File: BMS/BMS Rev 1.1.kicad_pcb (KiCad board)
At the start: 2 copper layers, 18 x 50.8 mm, 38 parts, among them J2 out, J3 out, J4 in, J5 in, Q1 CSD18502Q5B, Q2 CSD18502Q5B, U1 BQ41Z50RSNR

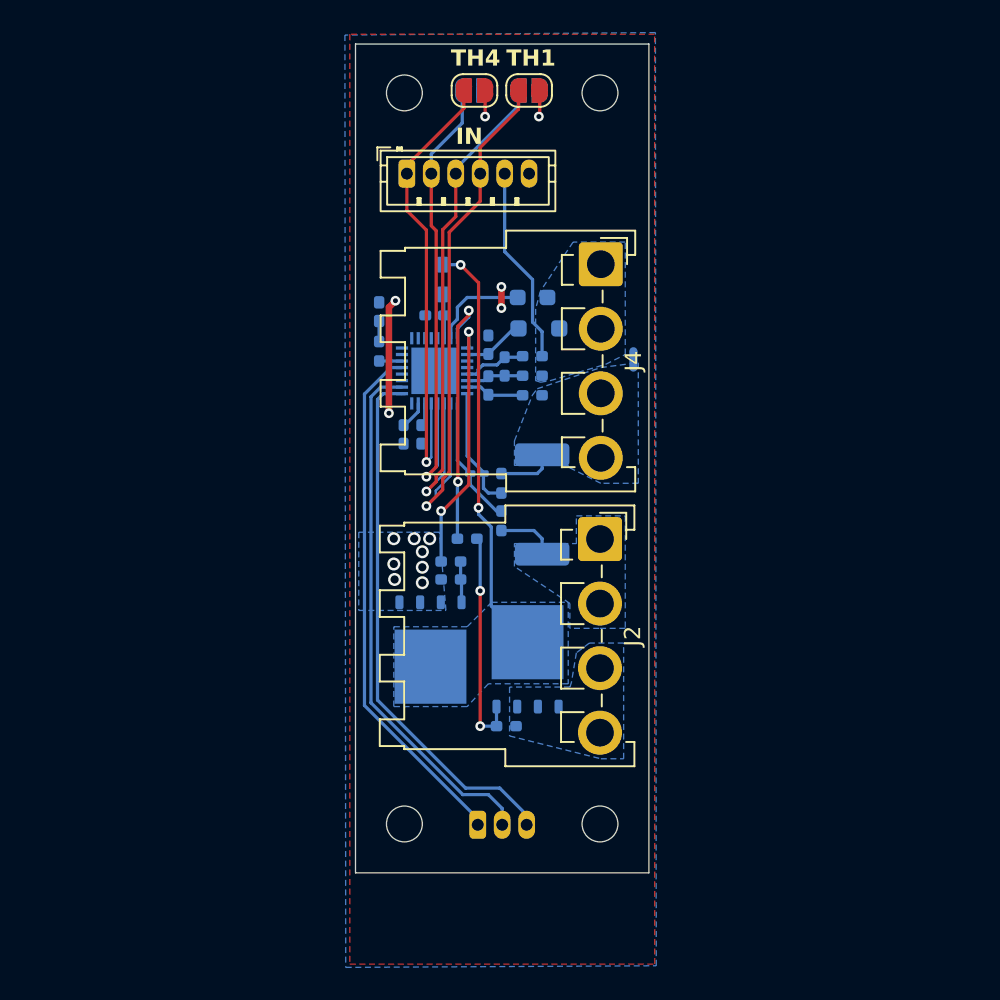
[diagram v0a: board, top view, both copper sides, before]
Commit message: Added everything
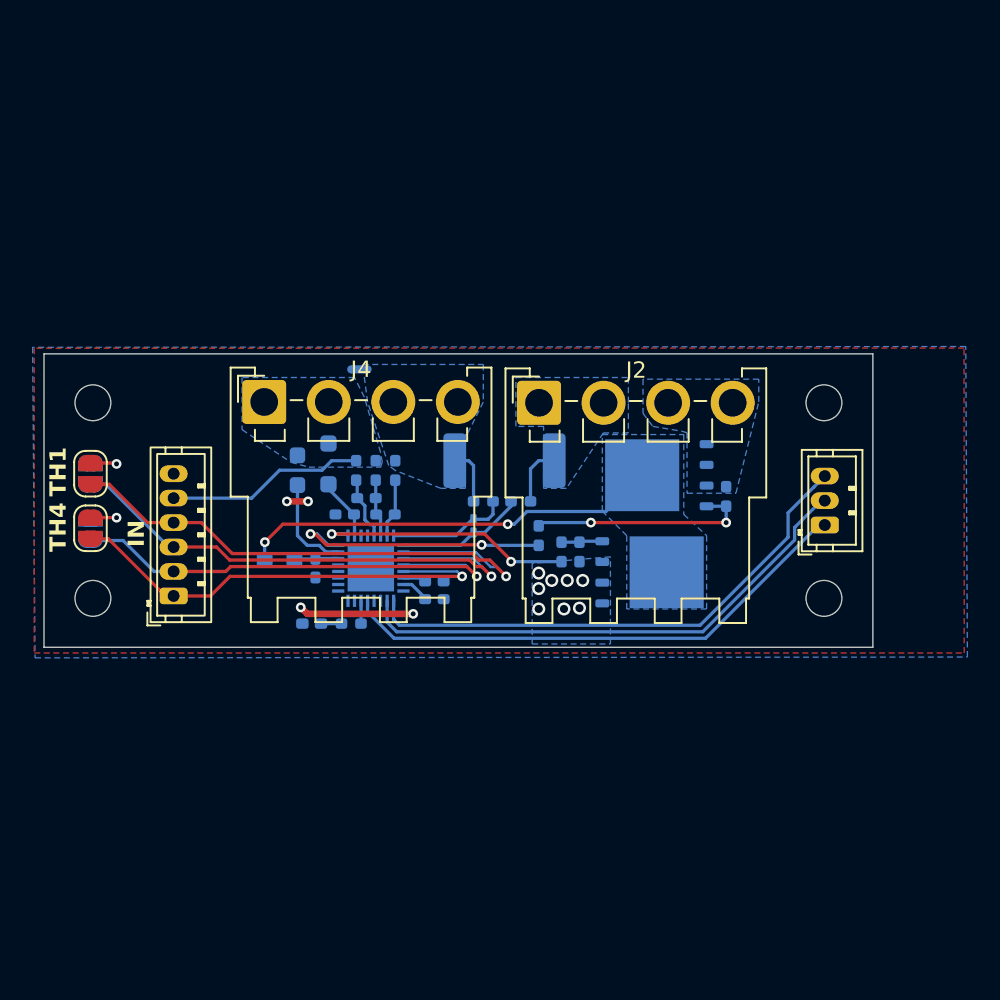
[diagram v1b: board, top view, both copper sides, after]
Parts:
- J3: moved to F.Cu
- moved REF** 36.5 mm to (149.9, 82.5), turned to 90 degrees
- moved REF** 36.4 mm to (149.9, 94.5), turned to 90 degrees
- moved JP3 35.7 mm to (149.7, 86.9), turned to 90 degrees
- moved JP4 35.7 mm to (149.7, 86.9), turned to 90 degrees
- moved JP2 35.7 mm to (149.7, 90.3), turned to 90 degrees
- moved JP1 35.7 mm to (149.7, 90.2), turned to 90 degrees
- moved J5 29.6 mm to (154.8, 94.4), turned to 90 degrees
- moved REF** 29.3 mm to (194.7, 82.5), turned to 90 degrees
- moved REF** 29.2 mm to (194.7, 94.5), turned to 90 degrees
- moved J3 28.1 mm to (194.8, 90.0), turned to 90 degrees
- moved J4 22.3 mm to (160.4, 82.5), turned to 0 degrees
- moved R6 19.9 mm to (161.3, 92.2), turned to 180 degrees
- moved D1 19.6 mm to (163.3, 96.1), turned to 0 degrees
- moved R8 19.5 mm to (188.7, 88.3), turned to -90 degrees
- moved R1 17.9 mm to (162.4, 86.6), turned to 90 degrees
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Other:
- board size 18 x 50.8 mm -> 50.9 x 18 mm
